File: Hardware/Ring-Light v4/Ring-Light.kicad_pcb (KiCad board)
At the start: 4 copper layers, 115 x 142.5 mm, 185 parts, among them U1 NCR321PASX, U10 NCR321PASX, U11 NCR321PASX, U12 NCR321PASX, U13 NCR321PASX, U14 NCR321PASX, U15 NCR321PASX, U16 NCR321PASX, U17 NCR321PASX, U18 NCR321PASX, U19 NCR321PASX, U2 NCR321PASX, U20 NCR321PASX, U21 NCR321PASX, U22 NCR321PASX, U23 NCR321PASX, U24 NCR321PASX, U25 NCR321PASX, U26 NCR321PASX, U27 NCR321PASX, U28 NCR321PASX, U29 NCR321PASX, U3 NCR321PASX, U30 NCR321PASX, U31 NCR321PASX, U32 NCR321PASX, U33 PCA9685BS,118, U4 NCR321PASX, U5 NCR321PASX, U6 NCR321PASX, U7 NCR321PASX, U8 NCR321PASX, U9 NCR321PASX

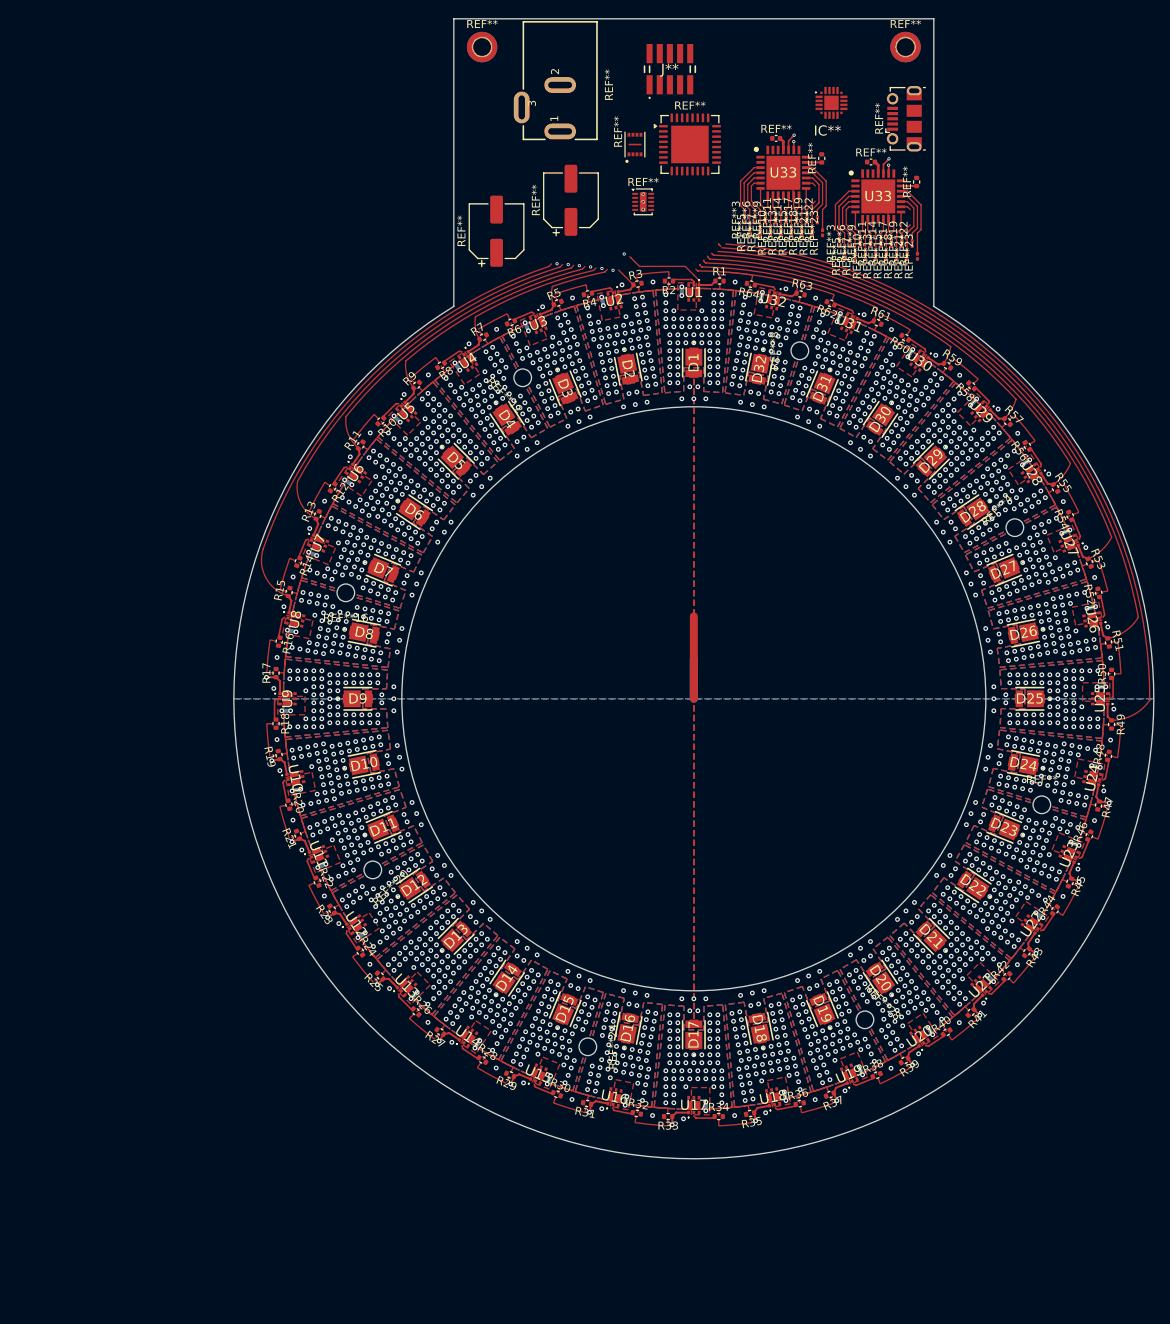
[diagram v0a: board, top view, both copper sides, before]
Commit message: m
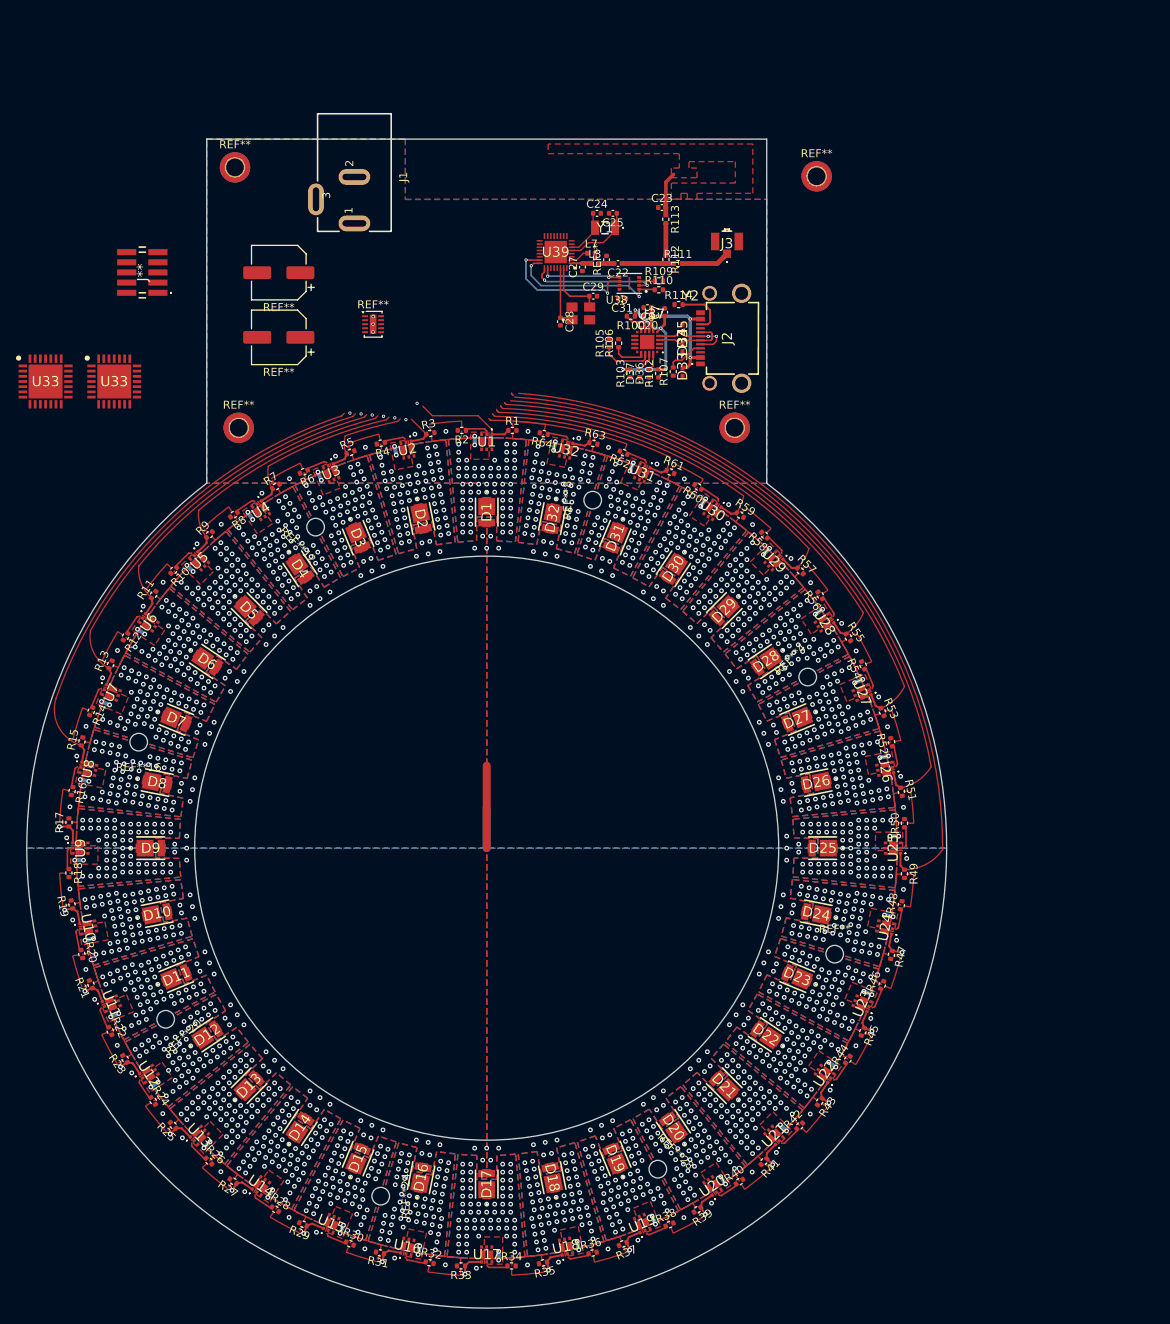
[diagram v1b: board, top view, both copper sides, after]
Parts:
- removed the REF** at (136.0, 32.5)
- removed the REF** at (147.8, 35.4)
- removed the REF** at (146.3, 27.5)
- removed the REF** at (119.5, 30.7)
- removed the REF** at (142.2, 32.9)
- removed the REF** at (130.3, 29.9)
- removed REF**10 (x2), REF**11 (x2), REF**13 (x2), REF**14 (x2), REF**15 (x2), REF**17 (x2), REF**18 (x2), REF**19 (x2), REF**21 (x2), REF**22 (x2), REF**23 (x2), REF**3 (x2), REF**5 (x2), REF**6 (x2), REF**7 (x2), REF**9 (x2): R_0201_0603Metric, Resistor_SMD:R_0201_0603Metric
- added C20: 1.0uF, Capacitor_SMD:C_0402_1005Metric, F.Cu at (114.2, 52.2)
- added C22: 12pF, Capacitor_SMD:C_0402_1005Metric, F.Cu at (110.5, 45.6)
- added C23: DNM, Capacitor_SMD:C_0402_1005Metric, F.Cu at (116.0, 38.6)
- added C24: 12pF, Capacitor_SMD:C_0402_1005Metric, F.Cu at (107.9, 39.3)
- added C25: 12pF, Capacitor_SMD:C_0402_1005Metric, F.Cu at (109.9, 39.3)
- added C27: 1.2pF, Capacitor_SMD:C_0402_1005Metric, F.Cu at (106.1, 46.0)
- added C28: DNM, Capacitor_SMD:C_0402_1005Metric, F.Cu at (103.3, 52.9)
- added C29: DNM, Capacitor_SMD:C_0402_1005Metric, F.Cu at (107.4, 49.7)
- added C31: 100nF, Capacitor_SMD:C_0402_1005Metric, F.Cu at (111.0, 50.0)
- added C7: 0.1uF, Capacitor_SMD:C_0402_1005Metric, F.Cu at (116.3, 51.7)
- added C8: 0.1uF, Capacitor_SMD:C_0402_1005Metric, F.Cu at (114.2, 51.1)
- added D33: TPD1E10B06DPYR, Library:TPD1E10B06DPYR, F.Cu at (118.6, 59.2)
- added D34: TPD1E10B06DPYR, Library:TPD1E10B06DPYR, F.Cu at (118.6, 56.1)
- added D35: TPD1E10B06DPYR, Library:TPD1E10B06DPYR, F.Cu at (118.6, 53.7)
- added D36: LTST-C170YKT, Diode_SMD:D_0402_1005Metric, F.Cu at (114.4, 59.3)
- added D37: LTST-C170YKT, Diode_SMD:D_0402_1005Metric, F.Cu at (113.2, 59.3)
- added J2: 1017457000B11LF, Library:1017457000B11LF, F.Cu at (124.5, 54.9)
- added J3: U.FL-R-SMT-1_80, Library:UFLRSMT180, F.Cu at (124.1, 42.8)
- added L3: 2nH, Inductor_SMD:L_0402_1005Metric, F.Cu at (107.6, 45.6)
- added L7: 15nH, Inductor_SMD:L_0402_1005Metric, F.Cu at (107.2, 44.3)
- added R100: 1k, Resistor_SMD:R_0402_1005Metric, F.Cu at (112.1, 52.2)
- added R102: 1k, Resistor_SMD:R_0402_1005Metric, F.Cu at (115.6, 59.3)
- added R103: 1k, Resistor_SMD:R_0402_1005Metric, F.Cu at (112.0, 59.3)
- added R105: 100k, Resistor_SMD:R_0402_1005Metric, F.Cu at (109.4, 55.5)
- added R106: 100k, Resistor_SMD:R_0402_1005Metric, F.Cu at (110.6, 55.5)
- added R107: 1k, Resistor_SMD:R_0402_1005Metric, F.Cu at (117.4, 59.1)
- added R109: 10k, Resistor_SMD:R_0402_1005Metric, F.Cu at (115.6, 47.8)
- added R110: 2.2k, Resistor_SMD:R_0402_1005Metric, F.Cu at (115.6, 48.9)
- added R111: DNM, Resistor_SMD:R_0402_1005Metric, F.Cu at (118.0, 45.6)
- added R112: 0, Resistor_SMD:R_0402_1005Metric, F.Cu at (116.5, 45.1)
- added R113: 0, Resistor_SMD:R_0402_1005Metric, F.Cu at (116.5, 40.1)
- added R114: 1k, Resistor_SMD:R_0402_1005Metric, F.Cu at (118.1, 50.7)
- added REF**: MountingHole_2.2mm_M2_DIN965_Pad_TopBottom, MountingHole:MountingHole_2.2mm_M2_DIN965_Pad_TopBottom, F.Cu at (125.1, 66.1)
- added REF**: C14, Capacitor_SMD:C_0402_1005Metric, F.Cu at (109.1, 45.1)
- added REF**: MountingHole_2.2mm_M2_DIN965_Pad_TopBottom, MountingHole:MountingHole_2.2mm_M2_DIN965_Pad_TopBottom, F.Cu at (63.1, 66.1)
- added U39: CC2640R2FRSMR, Library:QFN40P400X400X100-33N-D, F.Cu at (102.7, 44.2)
- added Y1: 32.768kHz, Library:FC135327680KAAG0, F.Cu at (108.9, 41.1)
- added Y2: 24MHz, Library:TSX-3225, F.Cu at (105.9, 51.8)
- U37: renamed from IC**; value CP2102NA02GQFN20 -> CP2102N-A02-GQFN20R
- U38: renamed from REF**; value PSON50P300X200X60-9N -> W25X40CLUXIG_TR
- moved U33 106.6 mm to (39.0, 60.3)
- moved U33 87.6 mm to (47.5, 60.3)
- moved J** 70.7 mm to (51.1, 46.7), turned to 90 degrees
- moved U37 37.7 mm to (114.2, 55.4), turned to 180 degrees
- moved REF** 37.6 mm to (68.1, 46.7), turned to 180 degrees
- moved REF** 37.1 mm to (79.9, 53.2)
- moved REF** 34.4 mm to (62.6, 33.6)
- moved R31 31.9 mm to (80.8, 169.3)
- moved R61 31.9 mm to (117.1, 71.7)
- moved D12 31.9 mm to (59.2, 142.0)
- moved D22 31.9 mm to (129.0, 142.0)
- moved D23 31.9 mm to (132.9, 134.7)
- moved D29 31.9 mm to (123.8, 89.0)
- moved D3 31.9 mm to (78.0, 79.9)
- moved R3 31.9 mm to (87.1, 66.8)
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- renumbered REF** to J1
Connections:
- net /OUT1 renamed /LEDs_1-16/OUT1
- net /OUT10 renamed /LEDs_1-16/OUT10
- net /OUT11 renamed /LEDs_1-16/OUT11
- net /OUT12 renamed /LEDs_1-16/OUT12
- net /OUT13 renamed /LEDs_1-16/OUT13
- net /OUT14 renamed /LEDs_1-16/OUT14
- net /OUT15 renamed /LEDs_1-16/OUT15
- net /OUT16 renamed /LEDs_1-16/OUT16
- net /OUT17 renamed /LEDs_17-32/OUT17
- net /OUT18 renamed /LEDs_17-32/OUT18
- net /OUT19 renamed /LEDs_17-32/OUT19
- net /OUT2 renamed /LEDs_1-16/OUT2
- net /OUT20 renamed /LEDs_17-32/OUT20
- net /OUT21 renamed /LEDs_17-32/OUT21
- net /OUT22 renamed /LEDs_17-32/OUT22
- net /OUT23 renamed /LEDs_17-32/OUT23
- net /OUT24 renamed /LEDs_17-32/OUT24
- net /OUT25 renamed /LEDs_17-32/OUT25
- net /OUT26 renamed /LEDs_17-32/OUT26
- net /OUT27 renamed /LEDs_17-32/OUT27
- net /OUT28 renamed /LEDs_17-32/OUT28
- net /OUT29 renamed /LEDs_17-32/OUT29
- net /OUT3 renamed /LEDs_1-16/OUT3
- net /OUT30 renamed /LEDs_17-32/OUT30
- net /OUT31 renamed /LEDs_17-32/OUT31
- net /OUT32 renamed /LEDs_17-32/OUT32
- net /OUT4 renamed /LEDs_1-16/OUT4
- net /OUT5 renamed /LEDs_1-16/OUT5
- net /OUT6 renamed /LEDs_1-16/OUT6
- net /OUT7 renamed /LEDs_1-16/OUT7
- net /OUT8 renamed /LEDs_1-16/OUT8
- net /OUT9 renamed /LEDs_1-16/OUT9
- net /REXT1 renamed /LEDs_1-16/REXT1
- net /REXT10 renamed /LEDs_1-16/REXT10
- net /REXT11 renamed /LEDs_1-16/REXT11
- net /REXT12 renamed /LEDs_1-16/REXT12
- net /REXT13 renamed /LEDs_1-16/REXT13
- net /REXT14 renamed /LEDs_1-16/REXT14
- net /REXT15 renamed /LEDs_1-16/REXT15
- net /REXT16 renamed /LEDs_1-16/REXT16
- net /REXT17 renamed /LEDs_17-32/REXT17
- net /REXT18 renamed /LEDs_17-32/REXT18
- net /REXT19 renamed /LEDs_17-32/REXT19
- net /REXT2 renamed /LEDs_1-16/REXT2
- net /REXT20 renamed /LEDs_17-32/REXT20
- net /REXT21 renamed /LEDs_17-32/REXT21
- net /REXT22 renamed /LEDs_17-32/REXT22
- net /REXT23 renamed /LEDs_17-32/REXT23
- net /REXT24 renamed /LEDs_17-32/REXT24
- net /REXT25 renamed /LEDs_17-32/REXT25
- net /REXT26 renamed /LEDs_17-32/REXT26
- net /REXT27 renamed /LEDs_17-32/REXT27
- net /REXT28 renamed /LEDs_17-32/REXT28
- net /REXT29 renamed /LEDs_17-32/REXT29
- net /REXT3 renamed /LEDs_1-16/REXT3
- net /REXT30 renamed /LEDs_17-32/REXT30
- net /REXT31 renamed /LEDs_17-32/REXT31
- net /REXT32 renamed /LEDs_17-32/REXT32
- net /REXT4 renamed /LEDs_1-16/REXT4
- net /REXT5 renamed /LEDs_1-16/REXT5
- net /REXT6 renamed /LEDs_1-16/REXT6
- net /REXT7 renamed /LEDs_1-16/REXT7
- net /REXT8 renamed /LEDs_1-16/REXT8
- net /REXT9 renamed /LEDs_1-16/REXT9
- net PWM1 renamed /LEDs_1-16/PWM1
- net PWM10 renamed /LEDs_1-16/PWM10
- net PWM11 renamed /LEDs_1-16/PWM11
- net PWM12 renamed /LEDs_1-16/PWM12
- net PWM13 renamed /LEDs_1-16/PWM13
- net PWM14 renamed /LEDs_1-16/PWM14
- net PWM15 renamed /LEDs_1-16/PWM15
- net PWM16 renamed /LEDs_1-16/PWM16
- net PWM17 renamed /LEDs_17-32/PWM17
- net PWM18 renamed /LEDs_17-32/PWM18
- net PWM19 renamed /LEDs_17-32/PWM19
- net PWM2 renamed /LEDs_1-16/PWM2
- net PWM20 renamed /LEDs_17-32/PWM20
- net PWM21 renamed /LEDs_17-32/PWM21
- net PWM22 renamed /LEDs_17-32/PWM22
- net PWM23 renamed /LEDs_17-32/PWM23
- net PWM24 renamed /LEDs_17-32/PWM24
- net PWM25 renamed /LEDs_17-32/PWM25
- net PWM26 renamed /LEDs_17-32/PWM26
- net PWM27 renamed /LEDs_17-32/PWM27
- net PWM28 renamed /LEDs_17-32/PWM28
- net PWM29 renamed /LEDs_17-32/PWM29
- net PWM3 renamed /LEDs_1-16/PWM3
- net PWM30 renamed /LEDs_17-32/PWM30
- net PWM31 renamed /LEDs_17-32/PWM31
- net PWM32 renamed /LEDs_17-32/PWM32
- net PWM4 renamed /LEDs_1-16/PWM4
- net PWM5 renamed /LEDs_1-16/PWM5
- net PWM6 renamed /LEDs_1-16/PWM6
- net PWM7 renamed /LEDs_1-16/PWM7
- net PWM8 renamed /LEDs_1-16/PWM8
- net PWM9 renamed /LEDs_1-16/PWM9
- net PWM_EN renamed /MCU/PWM_EN
- net SCL renamed /MCU/SCL
- net SDA renamed /MCU/SDA
- J1 pad 1: (no net) -> GND
- J1 pad 2: (no net) -> +12V
- J1 pad 3: (no net) -> unconnected-(J1-Pad3)
- U37 pad 1: (no net) -> unconnected-(U37-GPIO.1_/_RS485-Pad1)
- U37 pad 10: (no net) -> unconnected-(U37-NC-Pad10)
- U37 pad 11: (no net) -> unconnected-(U37-~{SUSPEND}-Pad11)
- U37 pad 12: (no net) -> GND
- U37 pad 13: (no net) -> unconnected-(U37-WAKEUP-Pad13)
- U37 pad 14: (no net) -> unconnected-(U37-SUSPEND-Pad14)
- U37 pad 15: (no net) -> unconnected-(U37-CTS-Pad15)
- U37 pad 16: (no net) -> unconnected-(U37-RTS-Pad16)
- U37 pad 17: (no net) -> Net-(U37-RXD)
- U37 pad 18: (no net) -> Net-(U37-TXD)
- U37 pad 19: (no net) -> Net-(U37-GPIO.3_/_RXT)
- U37 pad 2: (no net) -> unconnected-(U37-GPIO.0_/_CLK-Pad2)
- U37 pad 20: (no net) -> Net-(U37-GPIO.2_/_TXT)
- U37 pad 21: (no net) -> GND
- U37 pad 3: (no net) -> GND
- U37 pad 4: (no net) -> /Interface/D+
- U37 pad 5: (no net) -> /Interface/D-
- U37 pad 6: (no net) -> USB_VDD
- U37 pad 7: (no net) -> /Interface/<NO NET>
- U37 pad 8: (no net) -> /Interface/<NO NET>
- U37 pad 9: (no net) -> Net-(U37-~{RST})
- U38 pad 1: (no net) -> FLASH_CS
- U38 pad 2: (no net) -> MISO
- U38 pad 3: (no net) -> Net-(U38-~{WP})
- U38 pad 4: (no net) -> GND
- U38 pad 5: (no net) -> MOSI
- U38 pad 6: (no net) -> SCLK
- U38 pad 7: (no net) -> Net-(U38-~{HOLD})
- U38 pad 8: (no net) -> +3.3V
- U38 pad 9: (no net) -> GND
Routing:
- net FLASH_CS: track 0.00 -> 19.9 mm, vias 0 -> 2
- net USB_VDD: track 0.00 -> 19.9 mm, vias 0 -> 4
- net Net-(U33-LED15): track 19.0 -> 0.00 mm
- net /Interface/<NO NET>: track 0.00 -> 18.1 mm, vias 0 -> 3
- net SCLK: track 0.00 -> 17.8 mm, vias 0 -> 2
- net Net-(U33-LED1): track 17.6 -> 0.00 mm
- net Net-(U33-LED13): track 16.0 -> 0.00 mm
- net MISO: track 0.00 -> 15.9 mm, vias 0 -> 2
- net Net-(U33-LED0): track 15.9 -> 0.00 mm
- net Net-(U33-LED3): track 14.6 -> 0.00 mm
- net Net-(U33-LED14): track 14.4 -> 0.00 mm
- net Net-(U33-LED2): track 12.9 -> 0.00 mm
- net Net-(U33-LED12): track 11.3 -> 0.00 mm
- net Net-(U33-LED11): track 10.9 -> 0.00 mm
- net /Interface/D-: track 0.00 -> 10.3 mm, vias 0 -> 2
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- added copper zone on F.Cu, net (none)
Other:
- board size 115 x 142.5 mm -> 115 x 146.1 mm

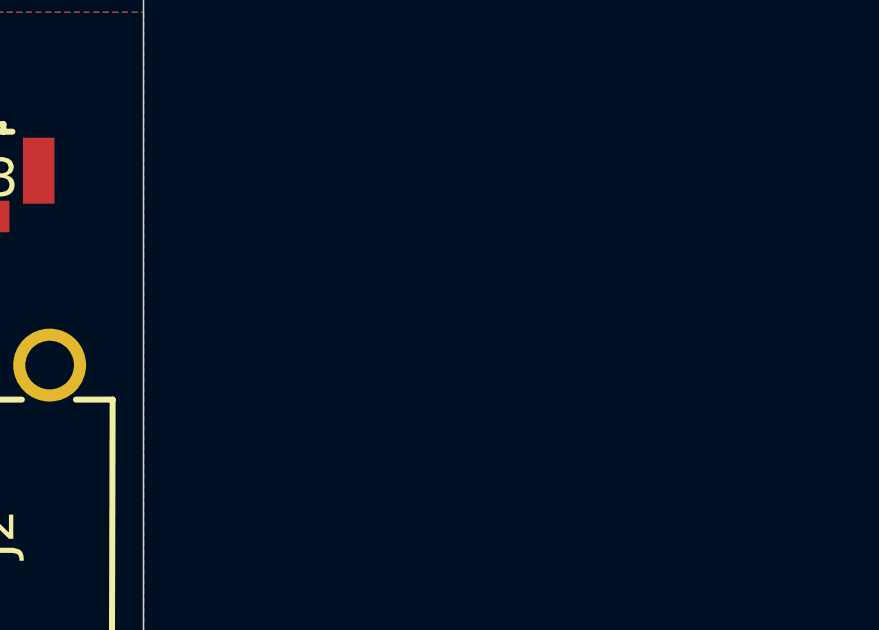
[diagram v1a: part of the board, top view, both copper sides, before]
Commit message: d
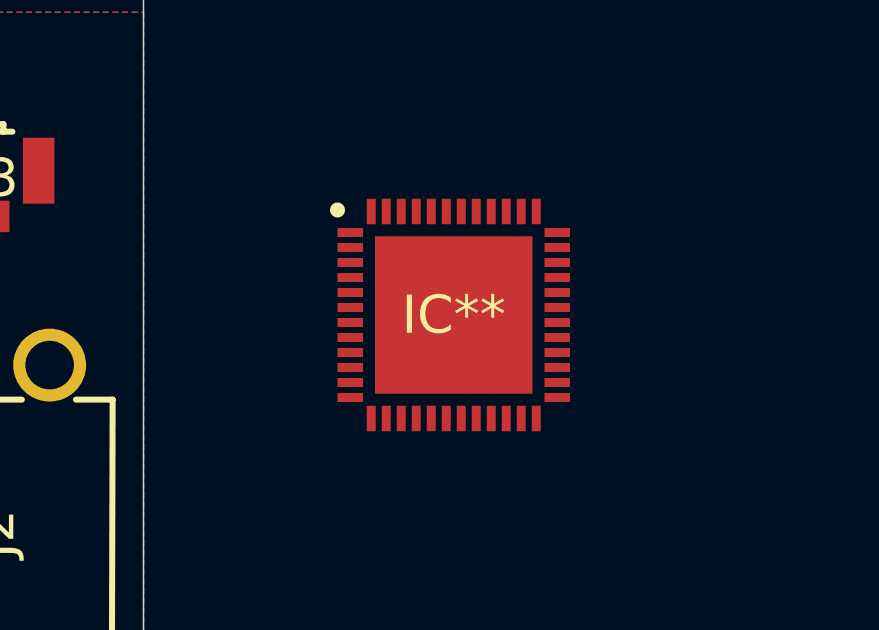
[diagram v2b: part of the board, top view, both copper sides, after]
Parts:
- added IC**: QFN50P700X700X100-49N-D, Library:QFN50P700X700X100-49N-D, F.Cu at (139.4, 47.6)
